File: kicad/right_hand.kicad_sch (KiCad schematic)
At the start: 29 parts, among them SW34 Gateron_ks_27, SW35 Gateron_ks_27, SW36 Gateron_ks_27, SW37 Gateron_ks_27, SW38 Gateron_ks_27, SW39 Gateron_ks_27, SW40 Gateron_ks_27, SW41 Gateron_ks_27, SW42 Gateron_ks_27, SW43 Gateron_ks_27, SW44 Gateron_ks_27, SW45 Gateron_ks_27, SW46 Gateron_ks_27, SW47 Gateron_ks_27, SW48 Gateron_ks_27, SW49 Gateron_ks_27, SW50 Gateron_ks_27, SW51 Gateron_ks_27, SW52 Gateron_ks_27, SW53 Gateron_ks_27, SW54 Gateron_ks_27, SW55 Gateron_ks_27, SW56 Gateron_ks_27, SW57 Gateron_ks_27, SW58 Gateron_ks_27, SW59 Gateron_ks_27, SW60 Gateron_ks_27, SW61 Gateron_ks_27, U3 74HC595

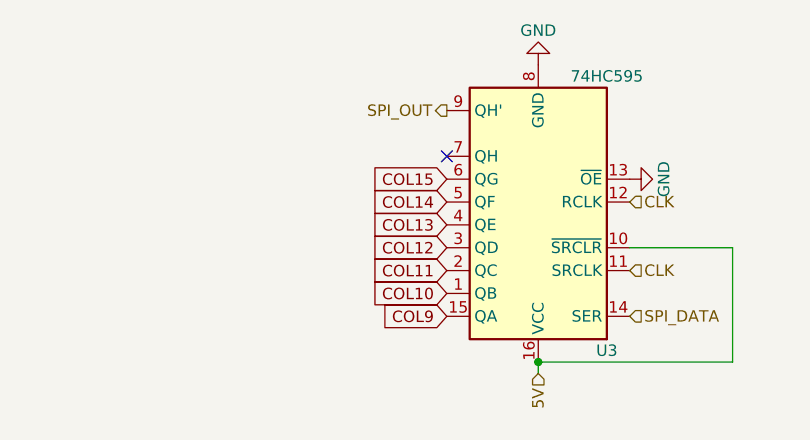
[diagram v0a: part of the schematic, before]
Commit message: Last update
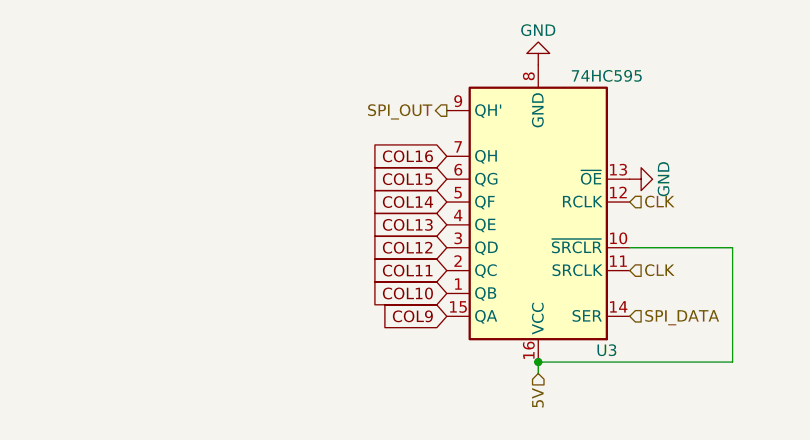
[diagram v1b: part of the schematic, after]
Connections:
- net COL16: now reaches U3.7 (QH)
- no-connect marks 1 -> 0
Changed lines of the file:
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@@
   (junction (at 161.29 125.73) (diameter 0) (color 0 0 0 0)
   )
-  (no_connect (at 194.31 60.96))
   (wire (pts (xy 201.93 110.49) (xy 201.93 105.41))
     (stroke (width 0) (type default) (color 0 0 0 0))
@@
     )
   )
+  (global_label "COL16" (shape input) (at 194.31 60.96 180) (fields_autoplaced)
+    (effects (font (size 1.27 1.27)) (justify right))
+    (property "Intersheet References" "${INTERSHEET_REFS}" (id 0) (at 185.8493 60.8806 0)
+      (effects (font (size 1.27 1.27)) (justify right) hide)
+    )
+  )
